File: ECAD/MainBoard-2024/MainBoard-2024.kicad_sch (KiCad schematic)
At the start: 60 parts, among them J1 XT60, J11 Conn_01x03, J12 Conn_01x04, J13 Conn_01x03, J14 Conn_01x03, J16 XT30, J17 XT30, J2 Conn_01x04, J20 BAU, J21 BAU, J22 Conn_01x04, J23 Conn_01x02, J26 BAU, J27 BAU, J28 Conn_01x02, J29 Conn_01x02, J3 ConStep1, J30 Conn_01x03, J5 ConStep1, J6 ConStep1, J7 XT30, J8 Conn_01x02, K1 CB1-P-24V, U1 Teensy3.5_All_Pins, U2 R-78B3.3-2.0, U3 R-78B12-2.0, U4 R-78B5.0-2.0

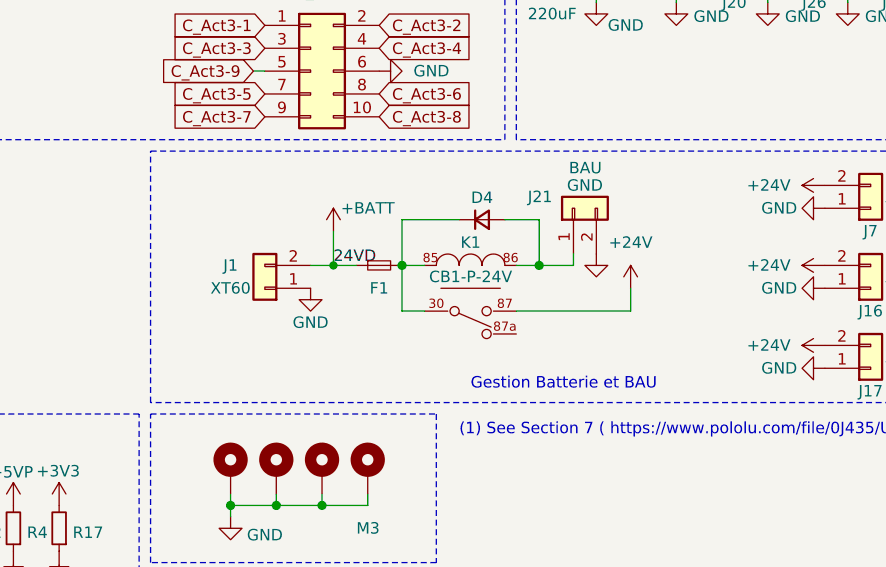
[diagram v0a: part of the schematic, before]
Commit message: change relay
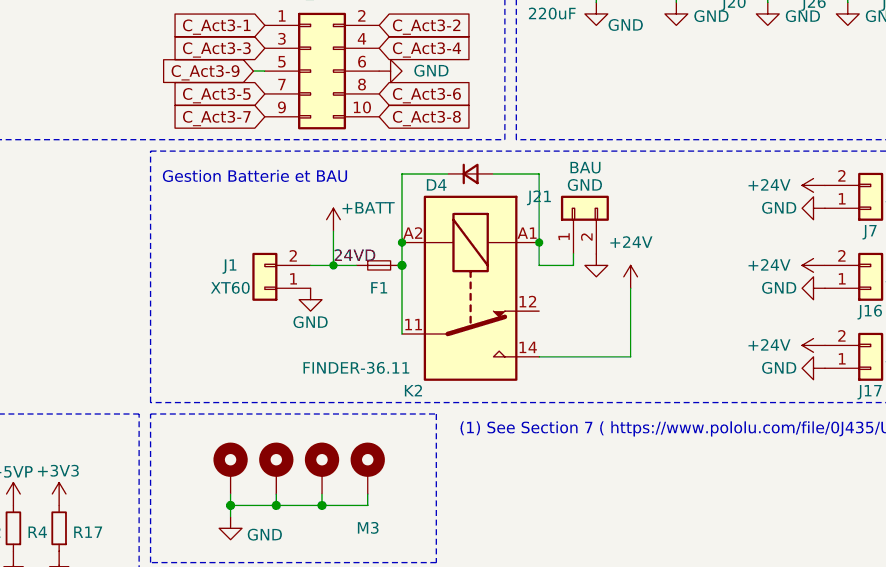
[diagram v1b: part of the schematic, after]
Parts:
- removed K1: CB1-P-24V, CB1-P-24V:Panasonic_Electric_Works-CB1-P-24V-MFG, symbol CB1-P-24V:CB1-P-24V
- added K2: FINDER-36.11, Relay_THT:Relay_SPDT_Finder_36.11, symbol Relay:FINDER-36.11
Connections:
- net +24V: now also K2.14
- net at D4.1 (K), F1.2: now also K2.11, K2.A2
- net at D4.2 (A), J21.1 (Pin_1): now also K2.A1
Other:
- moved on the sheet: D4
